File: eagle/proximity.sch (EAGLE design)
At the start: 13 parts

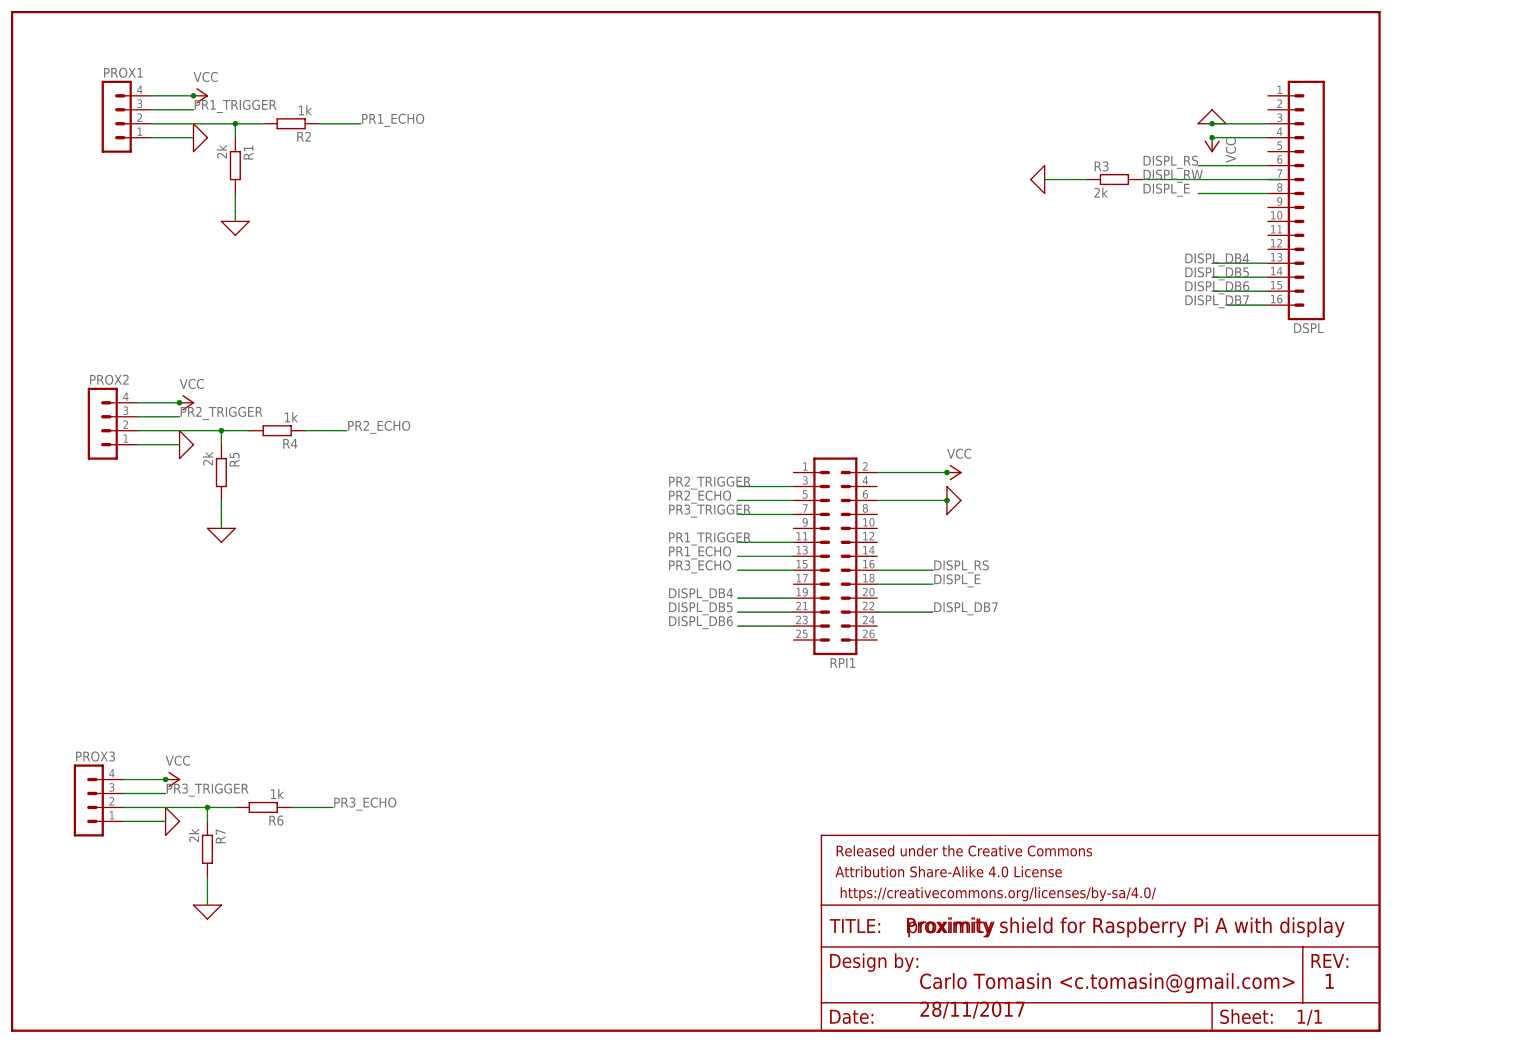
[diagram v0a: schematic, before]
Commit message: added PCB file
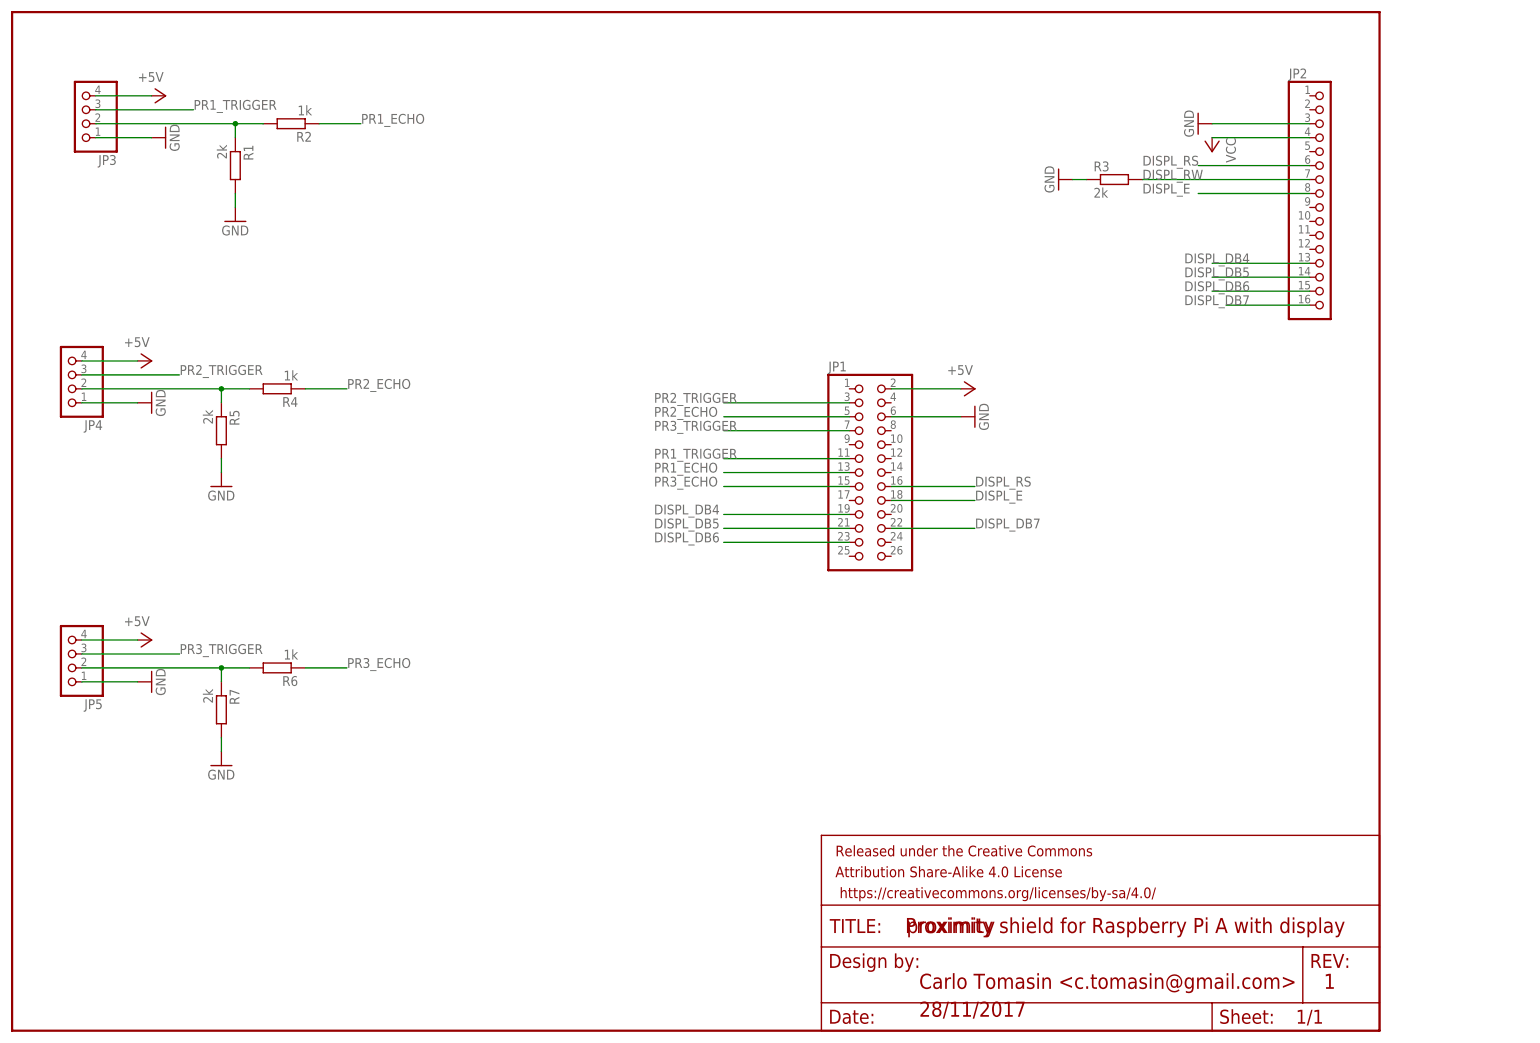
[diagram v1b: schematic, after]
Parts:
- removed DSPL: (no value), con-amp-quick:MA16
- removed PROX1, PROX2, PROX3: (no value), con-lstb:MA04-1
- removed RPI1: (no value), con-lstb:MA13-2
- added JP1: (no value), pinhead:PINHD-2X13
- added JP2: (no value), pinhead:PINHD-1X16
- added JP3, JP4, JP5: (no value), pinhead:PINHD-1X4
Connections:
- removed net 0: DSPL.3, PROX1.1, PROX2.1, PROX3.1, R1.2, R3.1, R5.2, R7.2, RPI1.6
- new net +5V: JP1.2, JP3.4, JP4.4, JP5.4
- new net GND: JP1.6, JP2.3, JP3.1, JP4.1, JP5.1, R1.2, R3.1, R5.2, R7.2
- net DISPL_DB4: now also JP1.19, JP2.13; no longer DSPL.13, RPI1.19
- net DISPL_DB5: now also JP1.21, JP2.14; no longer DSPL.14, RPI1.21
- net DISPL_DB6: now also JP1.23, JP2.15; no longer DSPL.15, RPI1.23
- net DISPL_DB7: now also JP1.22, JP2.16; no longer DSPL.16, RPI1.22
- net DISPL_E: now also JP1.18, JP2.8; no longer DSPL.8, RPI1.18
- net DISPL_RS: now also JP1.16, JP2.6; no longer DSPL.6, RPI1.16
- net DISPL_RW: now also JP2.7; no longer DSPL.7
- net N$1: now also JP3.2; no longer PROX1.2
- net N$2: now also JP4.2; no longer PROX2.2
- net N$3: now also JP5.2; no longer PROX3.2
- net PR1_ECHO: now also JP1.13; no longer RPI1.13
- net PR1_TRIGGER: now also JP1.11, JP3.3; no longer PROX1.3, RPI1.11
- net PR2_ECHO: now also JP1.5; no longer RPI1.5
- net PR2_TRIGGER: now also JP1.3, JP4.3; no longer PROX2.3, RPI1.3
- net PR3_ECHO: now also JP1.15; no longer RPI1.15
- net PR3_TRIGGER: now also JP1.7, JP5.3; no longer PROX3.3, RPI1.7
- net VCC: now also JP2.4; no longer DSPL.4, PROX1.4, PROX2.4, PROX3.4, RPI1.2
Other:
- moved on the sheet: R4, R5, R6, R7
